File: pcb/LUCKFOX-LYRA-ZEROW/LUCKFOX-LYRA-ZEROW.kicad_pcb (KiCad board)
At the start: 4 copper layers, 89.7 x 24.1 mm, 73 parts, among them J1 Conn_01x07, J2 Conn_01x05, J3 Conn_01x07, J4 Conn_01x05, J5 Conn_01x05, U1 Luckfox_Lyra_Zero_W, U10 RAA211403, U11 SN74LVC1G74DCUT, U12 74LVC2G66, U13 TPS3839G33DBZT, U14 74AUP2G34GW,125, U2 CORE52840, U3 MAX3051, U4 MCP2518FD-xQBB, U5 MAX3051, U6 MAX3051, U7 MCP2518FD-xQBB, U8 MAX3051, U9 74AUP2G34GW,125, Y4 Crystal_GND24_Small, Y5 Crystal_GND24_Small

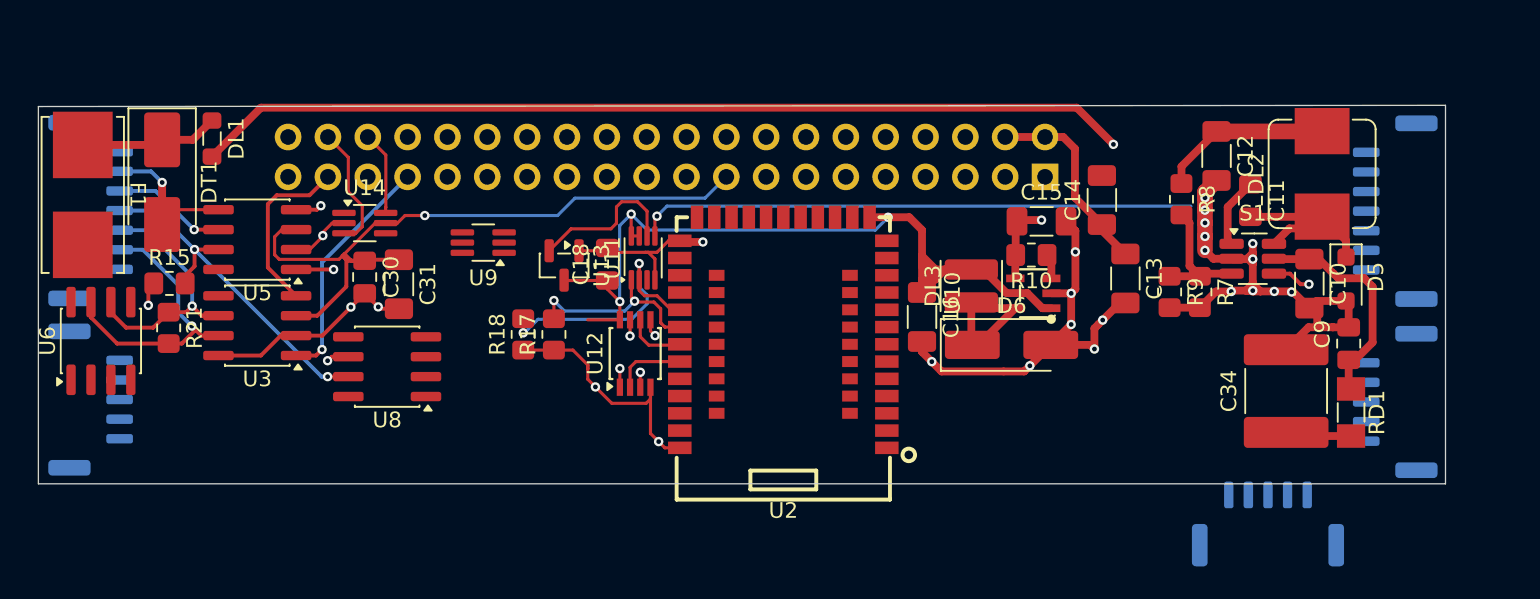
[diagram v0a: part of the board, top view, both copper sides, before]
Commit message: power pcb rework
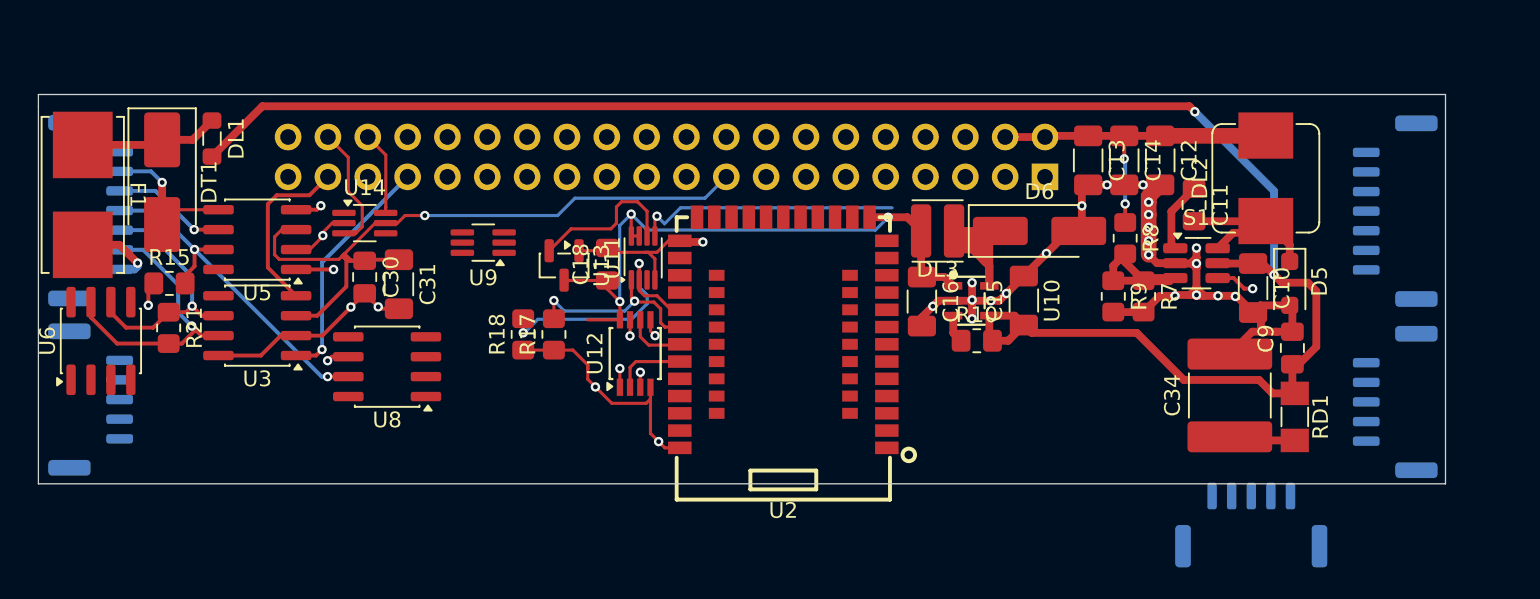
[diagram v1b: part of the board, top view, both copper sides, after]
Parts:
- moved C13 7.89 mm to (104.7, 44.2)
- moved D6 7.48 mm to (101.6, 48.7)
- moved R10 6.48 mm to (97.6, 55.7), turned to 0 degrees
- moved C15 5.17 mm to (100.6, 53.1), turned to 90 degrees
- moved R8 4.37 mm to (107.1, 49.2)
- moved DL3 4.11 mm to (95.1, 48.7), turned to 180 degrees
- moved U10 3.98 mm to (97.2, 53.1), turned to -90 degrees
- moved C11 3.60 mm to (111.5, 47.0)
- moved C12 3.60 mm to (109.3, 44.2)
- moved C9 3.60 mm to (117.7, 56.2)
- moved R7 3.60 mm to (108.2, 52.9)
- moved R9 3.60 mm to (106.3, 52.9)
- moved RD1 3.60 mm to (117.9, 60.6)
- moved C10 3.60 mm to (115.2, 52.3)
- moved S1 3.60 mm to (111.6, 50.8)
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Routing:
- net Net-(S1-Vin): track 86.6 -> 116.7 mm
- net /5V_EN: track 38.1 -> 19.4 mm
- net +3V3: track 57.6 -> 41.4 mm
- net Net-(D6-K): track 9.40 -> 19.9 mm
- net Net-(J1-Pin_1): track 0.00 -> 5.42 mm, vias 0 -> 1
- net GND: track 114.4 -> 110.6 mm, vias 25 -> 28
- net +5V: track 23.9 -> 21.8 mm, vias 0 -> 2
- net Net-(S1-FB): track 8.12 -> 10.0 mm
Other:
- board size 89.7 x 24.1 mm -> 89.7 x 24.8 mm
